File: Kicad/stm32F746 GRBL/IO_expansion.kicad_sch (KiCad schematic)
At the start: 4 parts, among them U1 MCP23008-xSO, U2 MCP23008-xSO

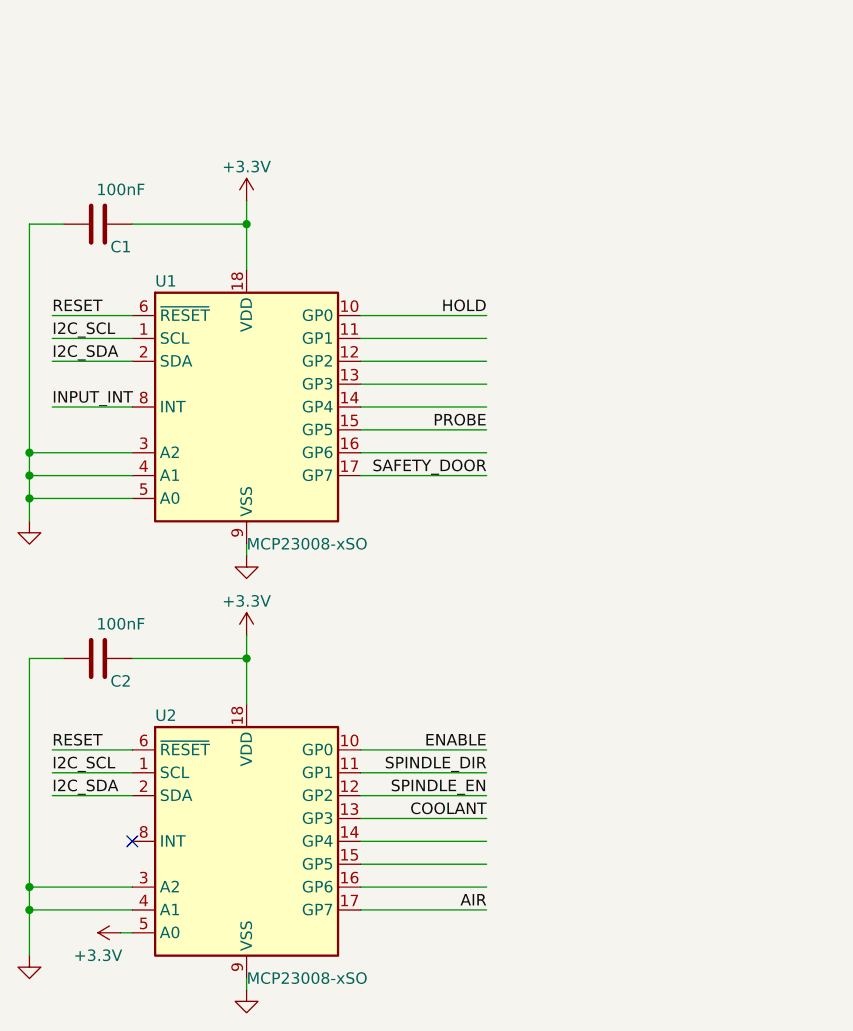
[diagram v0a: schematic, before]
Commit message: wip kicad
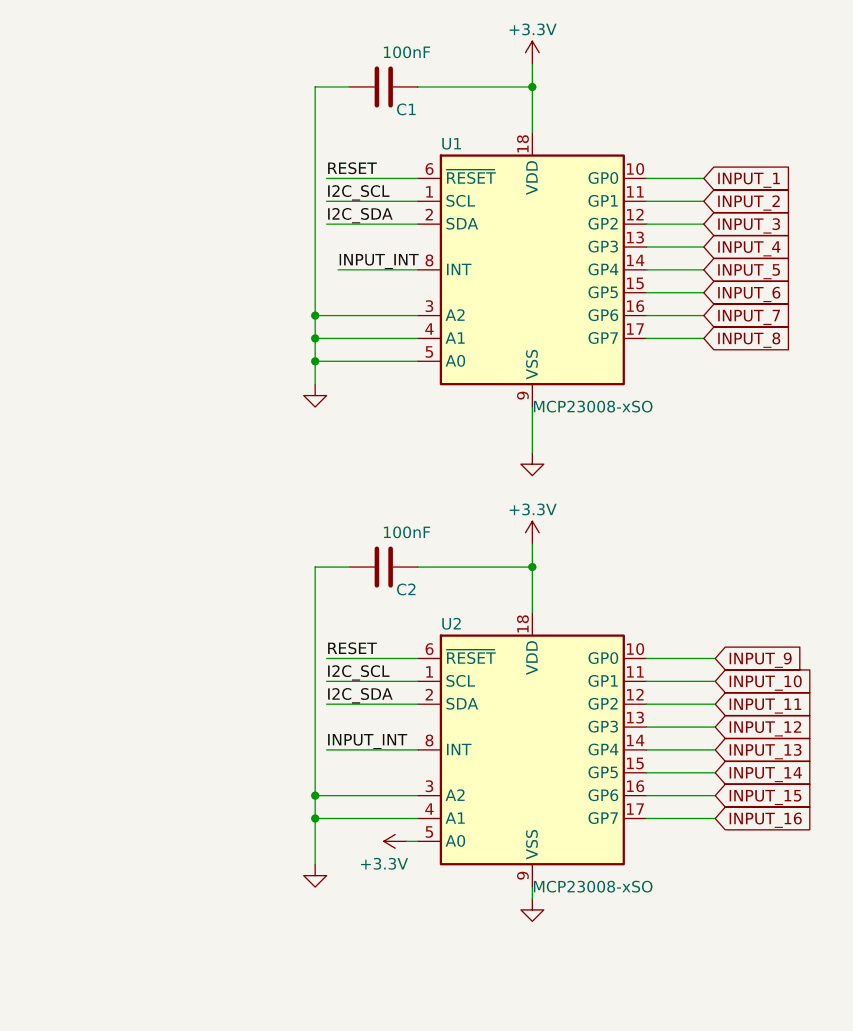
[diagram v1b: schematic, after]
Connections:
- net INPUT_INT: now also U2.8 (INT)
- net INPUT_13: now reaches U2.14 (GP4)
- net INPUT_14: now reaches U2.15 (GP5)
- net INPUT_15: now reaches U2.16 (GP6)
- net INPUT_2: now reaches U1.11 (GP1)
- net INPUT_3: now reaches U1.12 (GP2)
- net INPUT_4: now reaches U1.13 (GP3)
- net INPUT_5: now reaches U1.14 (GP4)
- net INPUT_7: now reaches U1.16 (GP6)
- net AIR renamed INPUT_16
- net COOLANT renamed INPUT_12
- net ENABLE renamed INPUT_9
- net HOLD renamed INPUT_1
- net PROBE renamed INPUT_6
- net SAFETY_DOOR renamed INPUT_8
- net SPINDLE_DIR renamed INPUT_10
- net SPINDLE_EN renamed INPUT_11
- no-connect marks 1 -> 0
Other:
- moved on the sheet: C1, C2, U1, U2

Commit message: wip Kicad
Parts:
- removed C1, C2: 100nF, Capacitor_SMD:C_0805_2012Metric, symbol Device:C
- removed U1, U2: MCP23008-xSO, Package_SO:SOIC-18W_7.5x11.6mm_P1.27mm, symbol Interface_Expansion:MCP23008-xSO
